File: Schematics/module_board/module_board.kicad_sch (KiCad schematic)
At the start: 2 parts, among them J1 Conn_01x06_Male

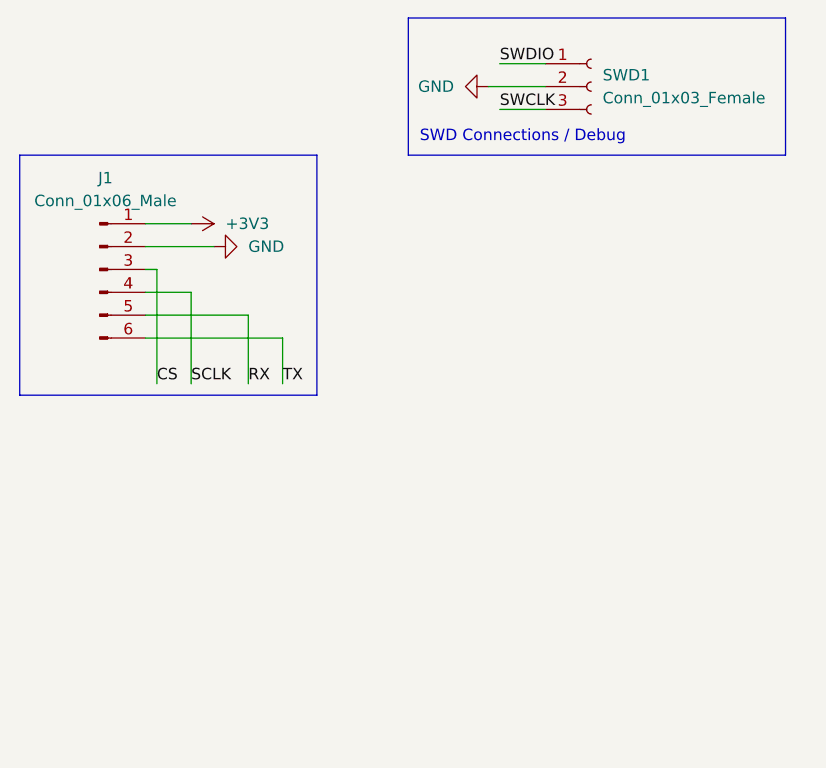
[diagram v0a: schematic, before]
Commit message: Added
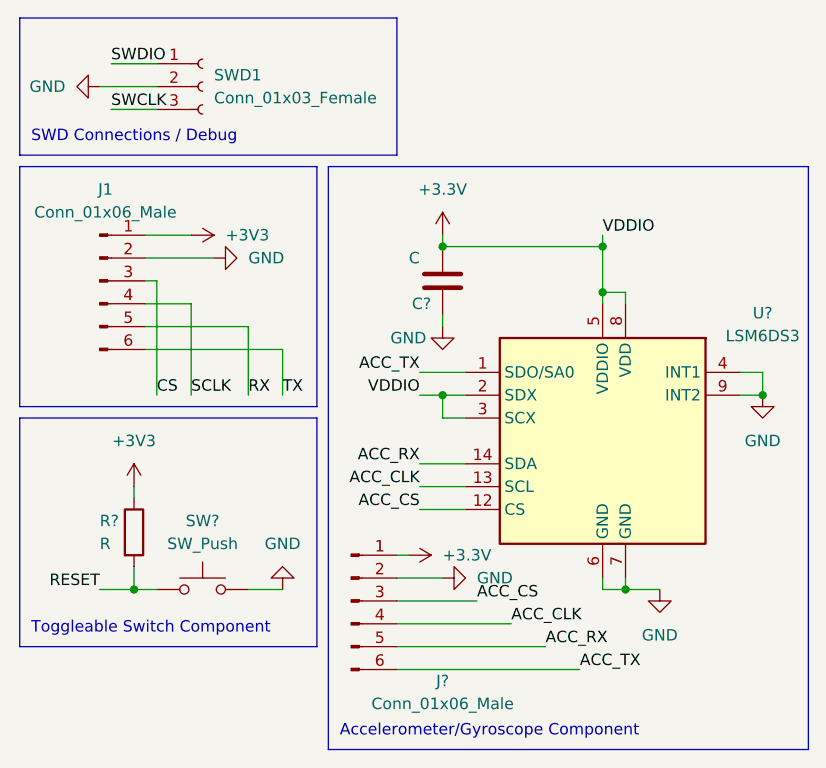
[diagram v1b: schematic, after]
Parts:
- added C?: C, symbol Device:C
- added J?: Conn_01x06_Male, symbol Connector:Conn_01x06_Male
- added R?: R, symbol Device:R
- added SW?: SW_Push, symbol Switch:SW_Push
- added U?: LSM6DS3, Package_LGA:LGA-14_3x2.5mm_P0.5mm_LayoutBorder3x4y, symbol Sensor_Motion:LSM6DS3
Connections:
- net +3V3: now also R?.1
- net GND: now also C?.1, J?.2 (Pin_2), SW?.2, U?.4 (INT1), U?.6 (GND), U?.7 (GND), U?.9 (INT2)
- new net +3.3V: C?.2, J?.1 (Pin_1), U?.2 (SDX), U?.3 (SCX), U?.5 (VDDIO), U?.8 (VDD)
- new net ACC_CLK: J?.4 (Pin_4), U?.13 (SCL)
- new net ACC_CS: J?.3 (Pin_3), U?.12 (CS)
- new net ACC_RX: J?.5 (Pin_5), U?.14 (SDA)
- new net ACC_TX: J?.6 (Pin_6), U?.1 (SDO/SA0)
- new net RESET: R?.2, SW?.1
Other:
- note added: "Accelerometer/Gyroscope Component"
- note added: "Toggleable Switch Component"
- moved on the sheet: J1, SWD1
